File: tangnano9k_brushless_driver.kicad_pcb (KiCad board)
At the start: 2 copper layers, 99.9 x 99.9 mm, 9 parts, among them J1 Nucleo_F302R8, J2 Conn_01x08_Socket, U1 Tang_Nano_9k_board, U2 MCP3008

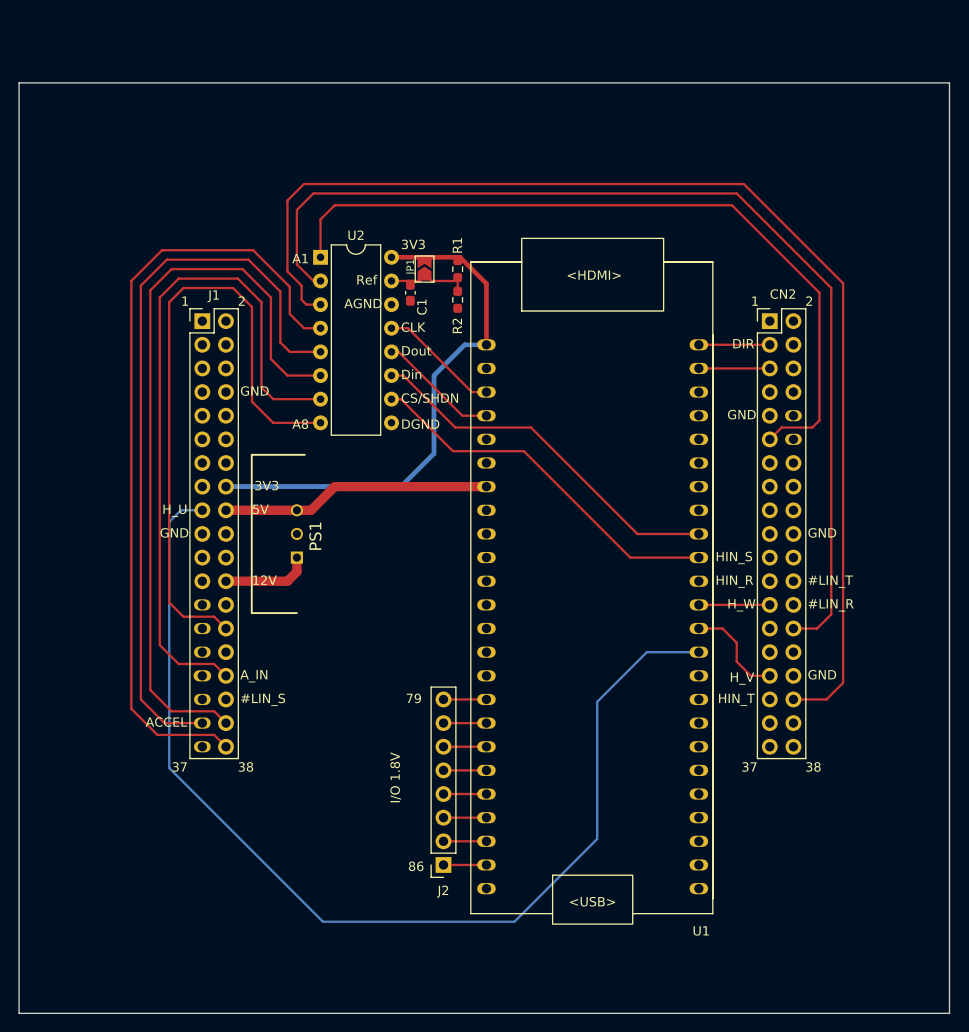
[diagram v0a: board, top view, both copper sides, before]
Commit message: 0908
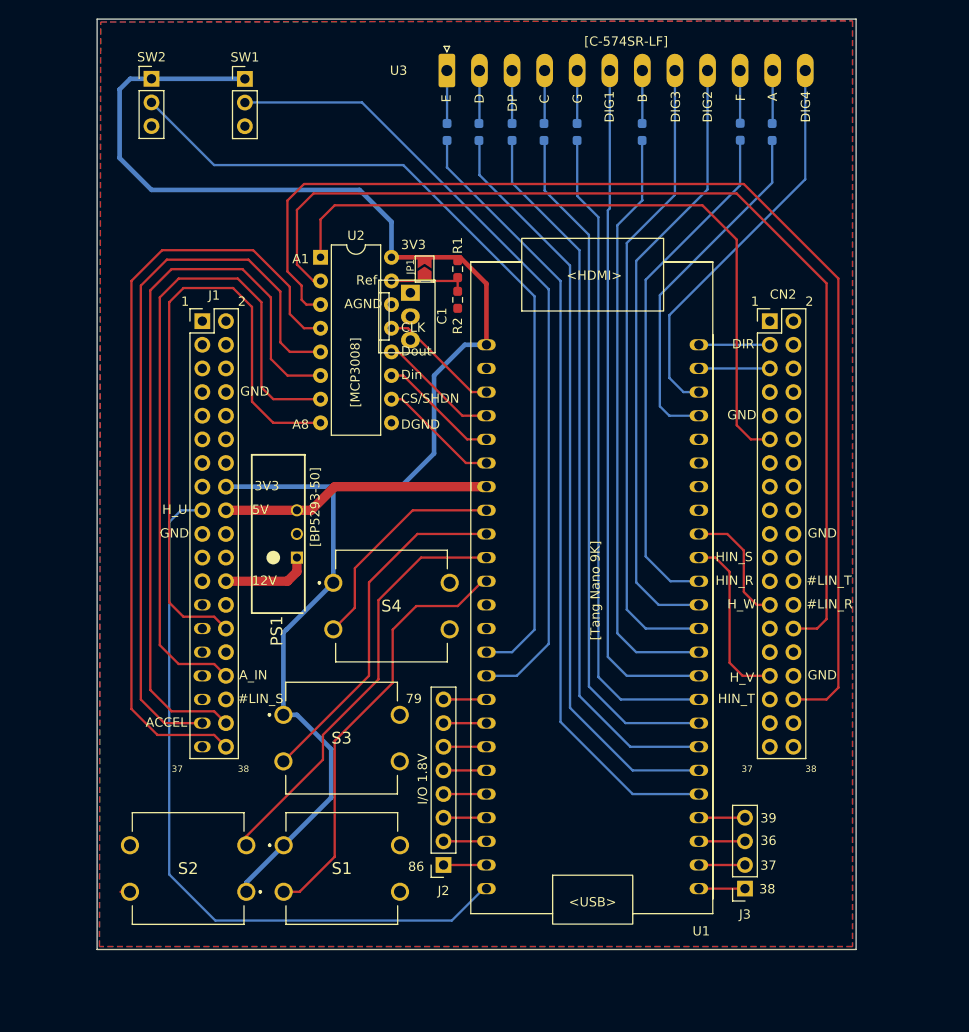
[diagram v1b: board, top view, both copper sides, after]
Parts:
- added J3: Conn_01x04_Socket, Connector_PinSocket_2.54mm:PinSocket_1x04_P2.54mm_Vertical, F.Cu at (187.8, 147.8)
- added R10: R, Resistor_SMD:R_0603_1608Metric_Pad0.98x0.95mm_HandSolder, B.Cu at (187.3, 66.5)
- added R3: R, Resistor_SMD:R_0603_1608Metric_Pad0.98x0.95mm_HandSolder, B.Cu at (155.8, 66.5)
- added R4: R, Resistor_SMD:R_0603_1608Metric_Pad0.98x0.95mm_HandSolder, B.Cu at (159.3, 66.5)
- added R5: R, Resistor_SMD:R_0603_1608Metric_Pad0.98x0.95mm_HandSolder, B.Cu at (162.8, 66.5)
- added R6: R, Resistor_SMD:R_0603_1608Metric_Pad0.98x0.95mm_HandSolder, B.Cu at (166.2, 66.5)
- added R7: R, Resistor_SMD:R_0603_1608Metric_Pad0.98x0.95mm_HandSolder, B.Cu at (169.8, 66.5)
- added R8: R, Resistor_SMD:R_0603_1608Metric_Pad0.98x0.95mm_HandSolder, B.Cu at (176.8, 66.5)
- added R9: R, Resistor_SMD:R_0603_1608Metric_Pad0.98x0.95mm_HandSolder, B.Cu at (190.8, 66.5)
- added S1: TVGP01-G73BB, samacsys:TVGP01G73BB, F.Cu at (138.3, 143.2)
- added S2: TVGP01-G73BB, samacsys:TVGP01G73BB, F.Cu at (134.3, 148.2)
- added S3: TVGP01-G73BB, samacsys:TVGP01G73BB, F.Cu at (138.2, 129.2)
- added S4: TVGP01-G73BB, samacsys:TVGP01G73BB, F.Cu at (143.6, 115.0)
- added SW1: SW_SPDT, Connector_PinHeader_2.54mm:PinHeader_1x03_P2.54mm_Vertical, F.Cu at (134.1, 60.8)
- added SW2: SW_SPDT, Connector_PinHeader_2.54mm:PinHeader_1x03_P2.54mm_Vertical, F.Cu at (124.1, 60.8)
- added U3: C-574SR-LF, Library:C-574SR-LF, F.Cu at (155.8, 59.9)
- C1: footprint Capacitor_SMD:C_0603_1608Metric_Pad1.08x0.95mm_HandSolder -> Connector:FanPinHeader_1x03_P2.54mm_Vertical
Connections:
- net +3.3V renamed +3V3
- U1 pad 1: unconnected-(U1-38/IOB31B/TF_CS-Pad1) -> Net-(J3-Pin_1)
- U1 pad 10: unconnected-(U1-30/IOB13B-Pad10) -> /DIG1
- U1 pad 11: /H_U -> Net-(U1-33/IOB23A/RGB_DE)
- U1 pad 12: /H_V -> /DIG3
- U1 pad 13: /H_W -> /DIG2
- U1 pad 14: unconnected-(U1-35/IOB29A/RGB_CK-Pad14) -> Net-(U1-35/IOB29A/RGB_CK)
- U1 pad 15: Net-(U1-41/IOB41A/RGB_B7) -> /H_V
- U1 pad 16: Net-(U1-42IOB41B/RGB_B6) -> /H_W
- U1 pad 2: unconnected-(U1-37/IO31A/TF_MOSI-Pad2) -> Net-(J3-Pin_2)
- U1 pad 21: unconnected-(U1-56/IOR14A/RGB_G6-Pad21) -> /Anode_A
- U1 pad 22: unconnected-(U1-57/IOR13A/RGB_G5-Pad22) -> /DIG4
- U1 pad 29: unconnected-(U1-49/IOR24A/SPILCD_RS-Pad29) -> /Din
- U1 pad 3: unconnected-(U1-36/IOB29B/TF_SCK-Pad3) -> Net-(J3-Pin_3)
- U1 pad 30: unconnected-(U1-48/IOR24B/SPILCD_CS-Pad30) -> /CS/SHDN
- U1 pad 32: unconnected-(U1-70/IOT41B/RGB_G2/HDMI_C0N-Pad32) -> Net-(S4-NO_1)
- U1 pad 33: unconnected-(U1-71/IOT41A/RGB_R7/HDMI_D0P-Pad33) -> Net-(S3-NO_1)
- U1 pad 34: unconnected-(U1-72/IOT39B/RGB_R6/HDMI_D1N-Pad34) -> Net-(S2-NO_1)
- U1 pad 35: unconnected-(U1-73/IOT39A/RGB_R5/HDMI_D1P-Pad35) -> Net-(S1-NO_1)
- U1 pad 38: unconnected-(U1-76/IOT37B/SPILCD_CK-Pad38) -> Net-(SW2-B)
- U1 pad 39: unconnected-(U1-77/IOT37A/SPILCD_MO-Pad39) -> Net-(SW1-B)
- U1 pad 4: unconnected-(U1-39/IOB33A/TF_MISO-Pad4) -> Net-(J3-Pin_4)
- U1 pad 48: unconnected-(U1-63/IOR5A/RGB_TOUCH_XL-Pad48) -> /H_U
- U1 pad 5: unconnected-(U1-25/IOB8A-Pad5) -> Net-(U1-25/IOB8A)
- U1 pad 6: unconnected-(U1-26/IOB8B-Pad6) -> Net-(U1-26/IOB8B)
- U1 pad 7: unconnected-(U1-27/IOB11A-Pad7) -> Net-(U1-27/IOB11A)
- U1 pad 8: unconnected-(U1-28/IOB11B-Pad8) -> Net-(U1-28/IOB11B)
- U1 pad 9: unconnected-(U1-29/IOB13A-Pad9) -> Net-(U1-29/IOB13A)
- U2 pad 10: Net-(U1-41/IOB41A/RGB_B7) -> /CS/SHDN
- U2 pad 11: Net-(U1-42IOB41B/RGB_B6) -> /Din
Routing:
- net +3V3: track 57.1 -> 166.9 mm
- net Net-(SW2-B): track 0.00 -> 91.8 mm
- net Net-(SW1-B): track 0.00 -> 87.0 mm
- net Net-(U1-25/IOB8A): track 0.00 -> 85.6 mm
- net Net-(U1-26/IOB8B): track 0.00 -> 81.6 mm
- net Net-(U1-27/IOB11A): track 0.00 -> 77.8 mm
- net Net-(U1-28/IOB11B): track 0.00 -> 74.1 mm
- net /DIG1: track 0.00 -> 73.7 mm
- net Net-(U1-29/IOB13A): track 0.00 -> 70.4 mm
- net /DIG3: track 0.00 -> 68.6 mm
- net /DIG2: track 0.00 -> 65.9 mm
- net Net-(U1-33/IOB23A/RGB_DE): track 0.00 -> 63.7 mm
- net Net-(U1-35/IOB29A/RGB_CK): track 0.00 -> 55.7 mm
- net Net-(S1-NO_1): track 0.00 -> 46.2 mm
- net Net-(S2-NO_1): track 0.00 -> 45.7 mm
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- added copper zone on B.Cu, net GND
- added copper zone on F.Cu, net GND
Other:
- board size 99.9 x 99.9 mm -> 81.5 x 99.9 mm
- board text added: "33"
- board text added: "34"
- board text added: "36"
- board text added: "39"
- board text added: "40"
- board text added: "41/H_V"
- board text added: "42/H_W"
- board text added: "48/CS SHDN"
- board text added: "49/Din"
- board text added: "51"
- board text added: "53"
- board text added: "54"
- board text added: "55"
- board text added: "63/H_U"
- board text added: "71"
- board text added: "72"
- board text added: "73"
- board text added: "75"
- board text added: "76"
- board text added: "A"
- board text added: "B"
- board text added: "C"
- board text added: "D"
- board text added: "DIG1"
- board text added: "DIG2"
- board text added: "DIG3"
- board text added: "DIG4"
- board text added: "DP"
- board text added: "E"
- board text added: "F"
- board text added: "G"
- board text added: "[BP5293-50]"
- board text added: "[C-574SR-LF]"
- board text added: "[MCP3008]"
- board text added: "[Tang Nano 9K]"
- board text removed: "33/H_U"
- board text removed: "34/H_V"
- board text removed: "40/H_W"
- board text removed: "41/CS SHDN"
- board text removed: "42/Din"
- board text removed: "48"
- board text removed: "49"
- board text removed: "63"
